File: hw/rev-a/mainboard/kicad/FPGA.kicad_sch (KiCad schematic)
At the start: 46 parts, among them J17 PMOD1, J18 PMOD2, J22 PROG, J4 BUS_EXPANSION, J9 FPGA_MCU, Q1 MMBT3904, SW3 CONFIG, U10 T20Q144C3

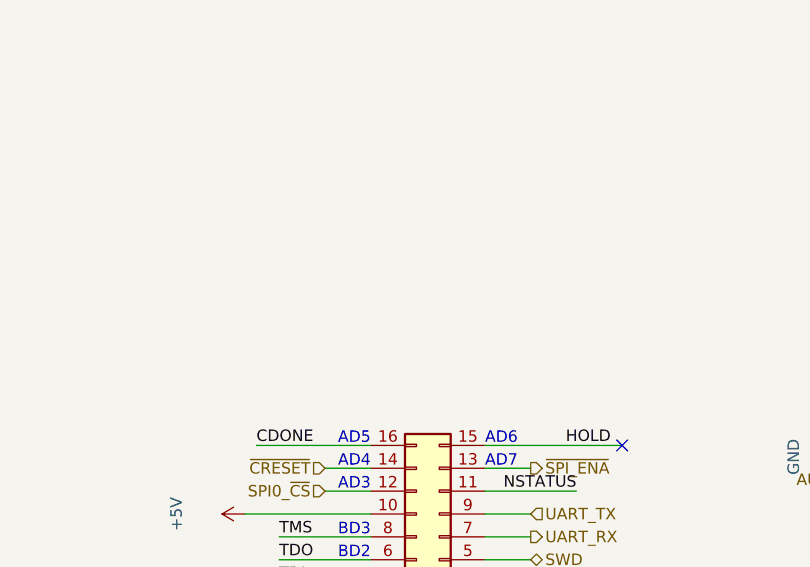
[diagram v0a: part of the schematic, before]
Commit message: hw: tidy schematics for publication
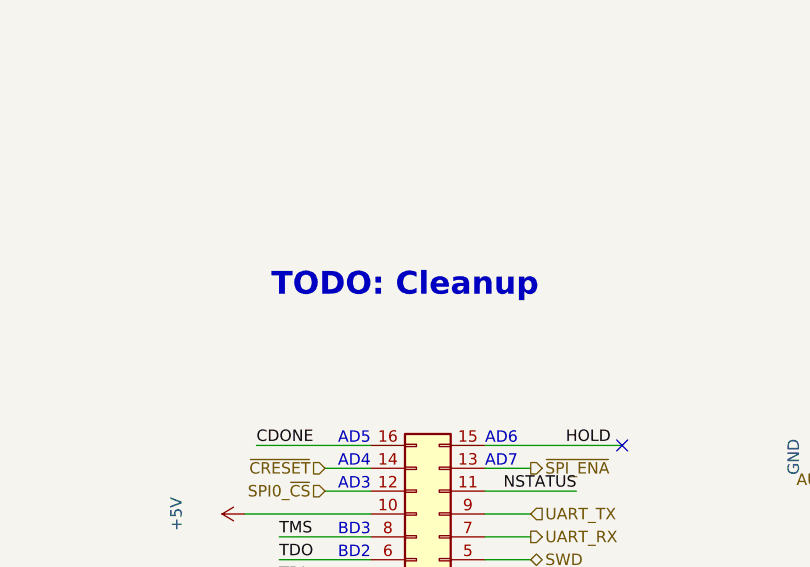
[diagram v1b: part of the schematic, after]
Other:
- note added: "TODO: Cleanup"
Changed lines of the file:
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@@
 		(date "2023-10-01")
 		(rev "A")
+		(comment 1 "Unspecified resistors are 1% and rated for 62.5mW or higher")
+		(comment 2 "Unspecified capacitors are rated for 25V or higher")
+		(comment 3 "Signals with B-prefix are level-shifted from 3V3 to 5V")
 	)
 	(junction
@@
 		)
 	)
+	(text "TODO: Cleanup"
+		(exclude_from_sim no)
+		(at 144.78 24.13 0)
+		(effects
+			(font
+				(size 2.54 2.54)
+				(thickness 0.508)
+				(bold yes)
+			)
+		)
+	)

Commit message: hw: tidy schematics for publication
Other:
- company: (none) -> https://is.gd/6hpvh6
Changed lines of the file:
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@@
 		(date "2023-10-01")
 		(rev "A")
-		(comment 1 "Unspecified resistors are 1% and rated for 62.5mW or higher")
-		(comment 2 "Unspecified capacitors are rated for 25V or higher")
+		(company "https://is.gd/6hpvh6")
+		(comment 1 "Unspecified resistors are 1% / 62.5mW")
+		(comment 2 "Unspecified capacitors are 25V")
 		(comment 3 "Signals with B-prefix are level-shifted from 3V3 to 5V")
+		(comment 4 "License: CC0 1.0 Universal (Public Domain Dedication)")
 	)
 	(junction
